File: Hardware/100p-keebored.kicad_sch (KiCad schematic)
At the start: 28 parts, among them J1 AVR-ISP-6, J2 USB_C_Receptacle_USB2.0, J3 Type C 31-M-12, J4 Conn_01x04, SW130 RotaryEncoder_Switch, SW200 SW_Push, U1 AT90USB1286-A, Y1 JYJE 3TJ480000JYLBC

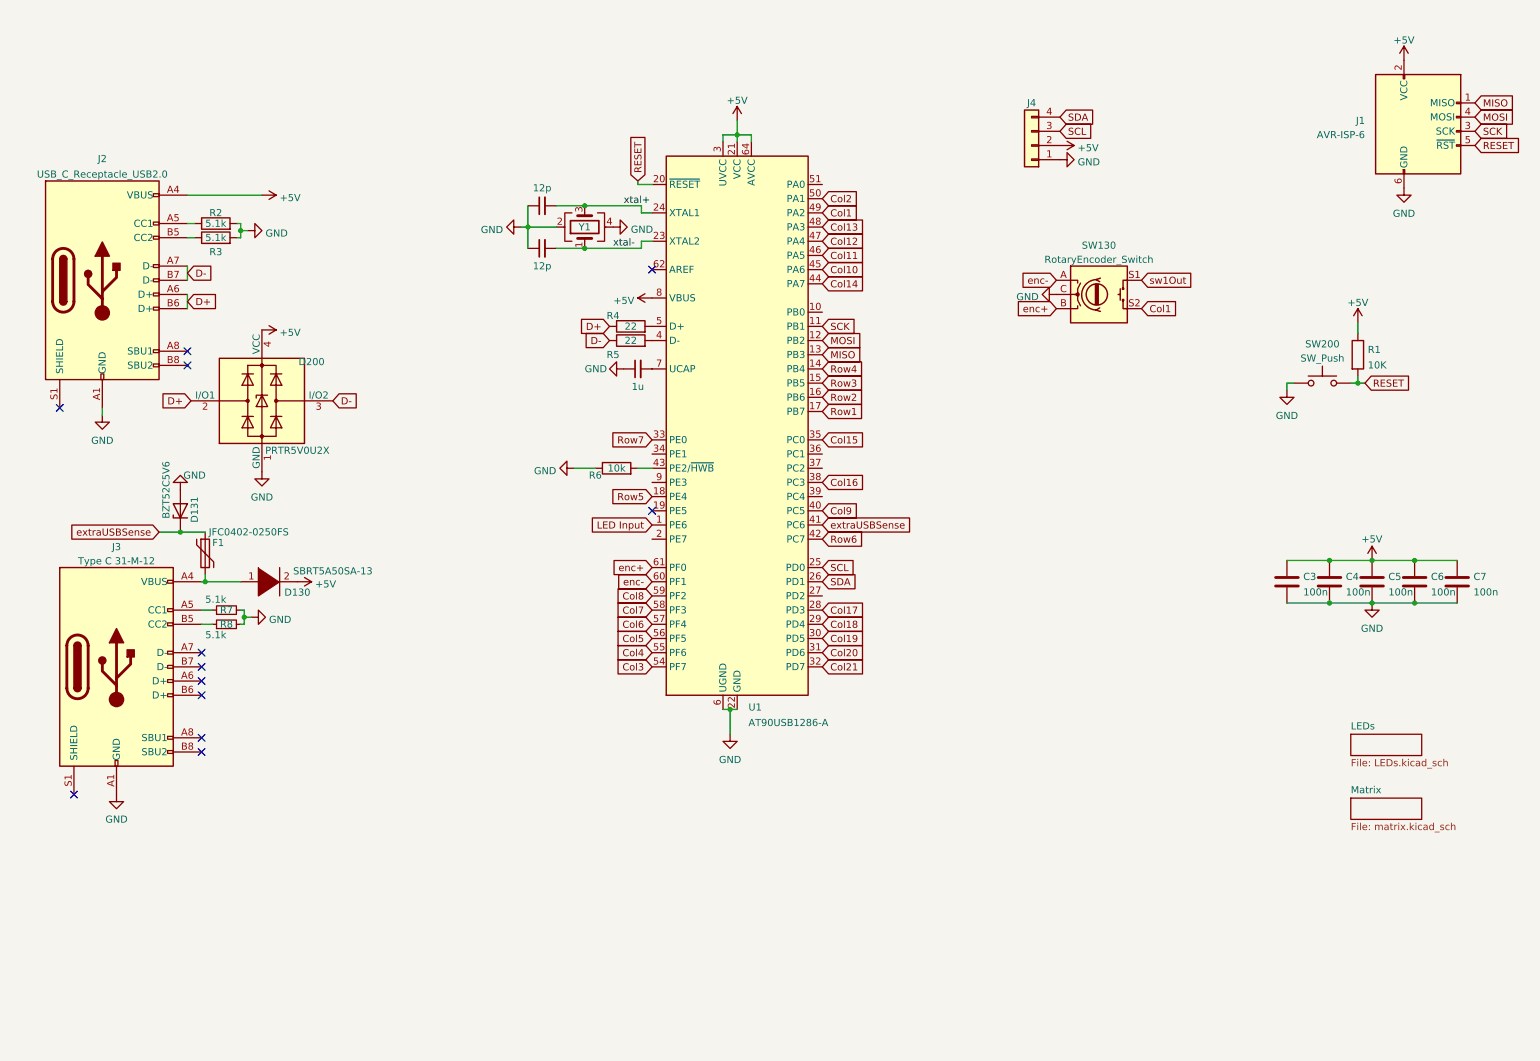
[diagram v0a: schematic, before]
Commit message: Final design for v2.0
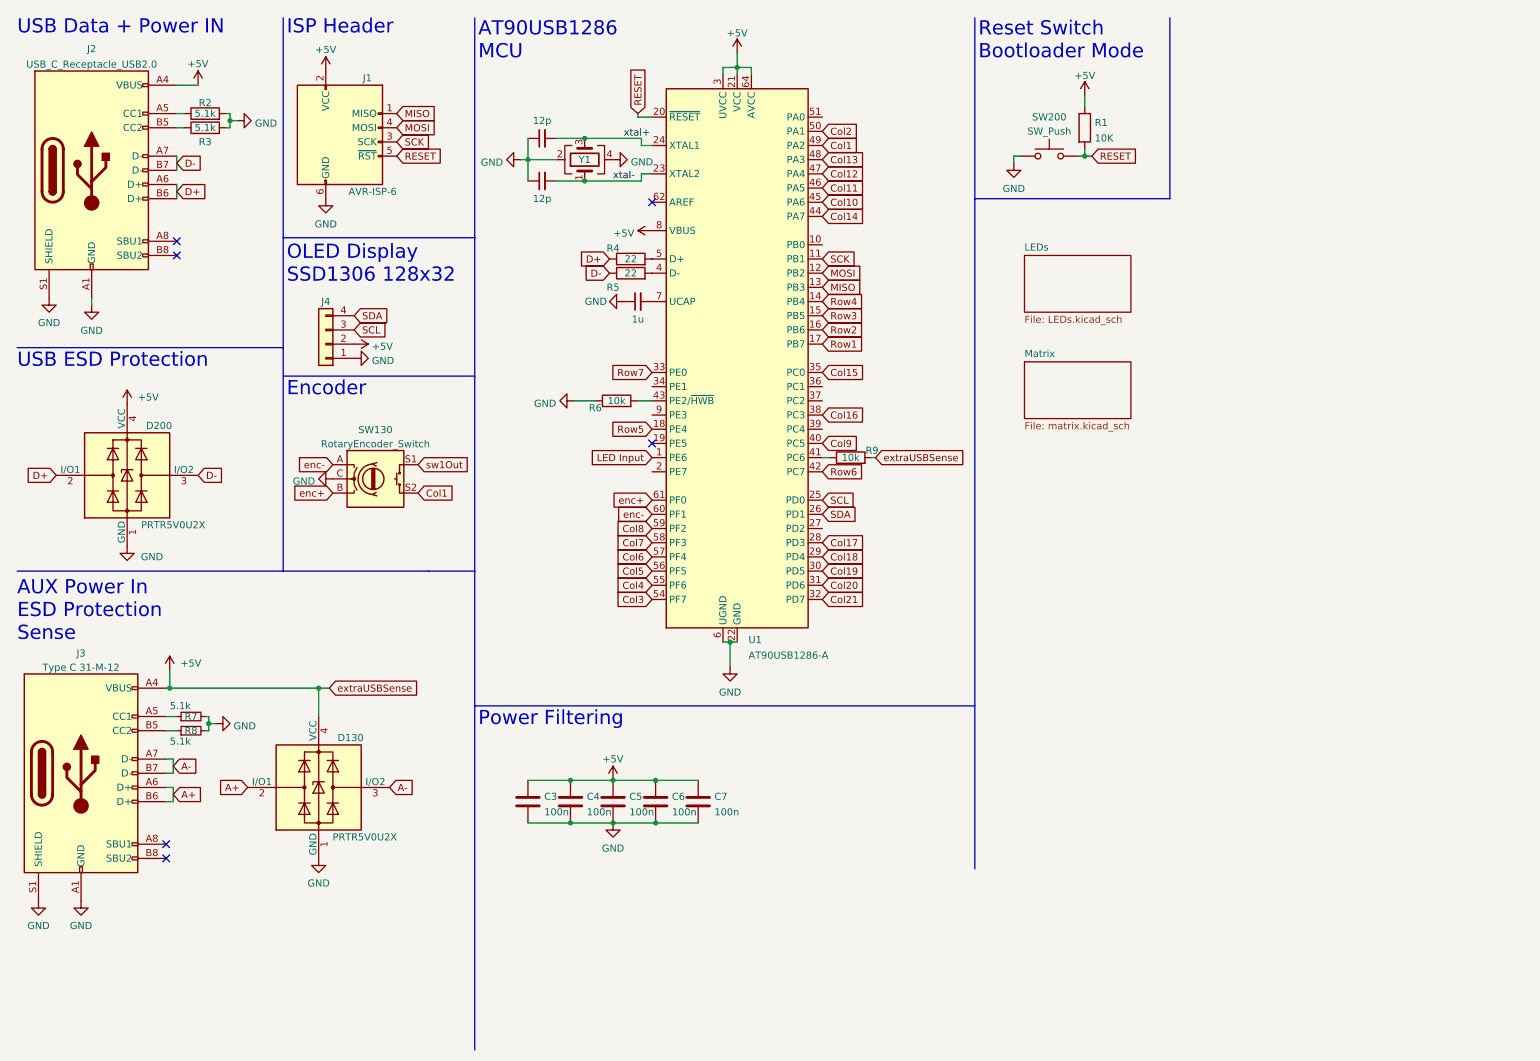
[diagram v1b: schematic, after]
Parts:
- removed D130: SBRT5A50SA-13, Diode_SMD:D_SMA, symbol pspice:DIODE
- removed D131: BZT52C5V6, Diode_SMD:D_SOD-123, symbol Device:D_Zener
- removed F1: JFC0402-0250FS, Fuse:Fuse_0402_1005Metric, symbol Device:Polyfuse
- added D130: PRTR5V0U2X, Package_TO_SOT_SMD:SOT-143, symbol Power_Protection:PRTR5V0U2X
- added R9: 10k, Resistor_SMD:R_0402_1005Metric, symbol Device:R
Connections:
- net +5V: now also J3.A4 (VBUS), J3.A9 (VBUS), J3.B4 (VBUS), J3.B9 (VBUS), D130.4 (VCC), R9.2
- net GND: now also J2.S1 (SHIELD), J3.S1 (SHIELD), D130.1 (GND)
- net A+: now reaches J3.A6 (D+)
- net A+: now also J3.B6 (D+), D130.2 (I/O1)
- net A-: now reaches J3.A7 (D-)
- net A-: now also J3.B7 (D-), D130.3 (I/O2)
- net extraUSBSense: no longer names the net of U1.41 (PC6)
- net extraUSBSense: now also R9.1
- no-connect marks 12 -> 6
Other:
- note added: "AT90USB1286 MCU"
- note added: "AUX Power In ESD Protection Sense"
- note added: "Encoder"
- note added: "ISP Header"
- note added: "OLED Display SSD1306 128x32"
- note added: "Power Filtering"
- note added: "Reset Switch Bootloader Mode"
- note added: "USB Data + Power IN"
- note added: "USB ESD Protection"
- moved on the sheet: C3, C4, C5, C6, C7, D200, J1, J2, J3, J4, R1, R2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
